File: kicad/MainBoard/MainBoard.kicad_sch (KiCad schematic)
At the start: 97 parts, among them J1 CHAN1, J10 ACC Port, J11 433TX, J12 VDC INPUT, J13 BAT, J14 TRG1, J15 TRG2, J16 FP-BUTTONS, J17 EXPAN2, J18 OUTPUT_BOARD_POWER, J19 FrontPanel, J2 CHAN2, J20 I2C, J21 EXPAN3, J3 OUTPUT_BOARD_IO, J4 OUTPUT_BOARD_FP, J5 CHAN4, J6 LCD, J7 CHAN3, J8 EXPAN1, J9 AudioJack3_SwitchTR, SW1 SW_SPST, U1 AT24C04C-PUM, U2 UT232A, U3 LM2941T, U4 Pico, U5 L78L33ACZTR, U6 LM2576T-5, U7 PCF8574, U8 PCF8574

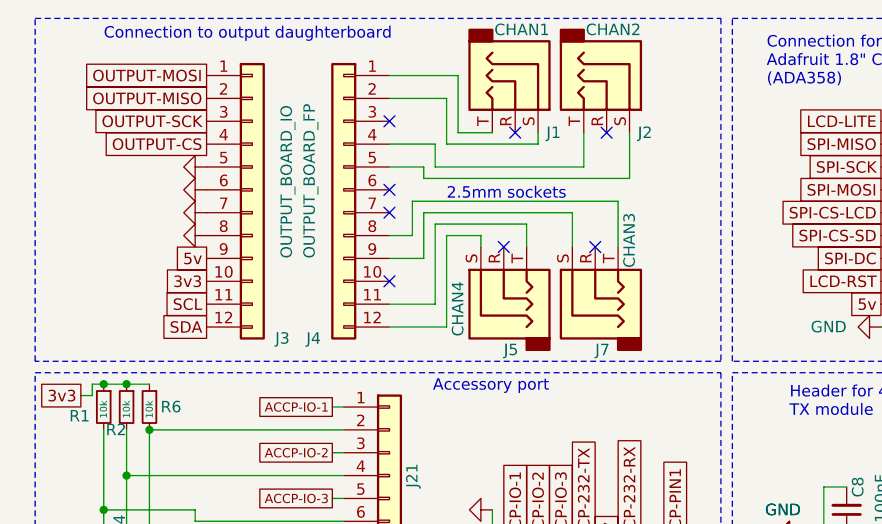
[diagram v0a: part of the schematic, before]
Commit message: Before 3.5mm footprint switch
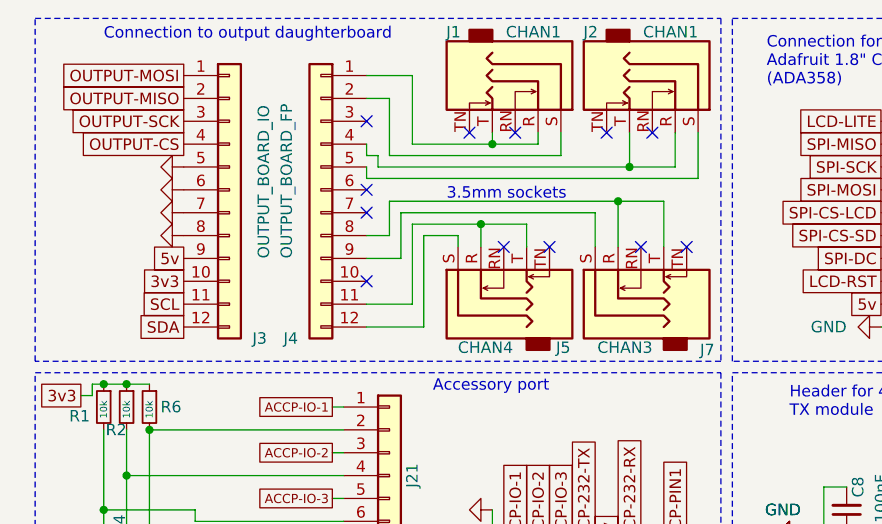
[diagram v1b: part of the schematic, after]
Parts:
- removed J1: CHAN1, ProjLib:PJ-2100B-4A, symbol MainBoard-rescue:AudioJack3-Connector
- removed J2: CHAN2, ProjLib:PJ-2100B-4A, symbol MainBoard-rescue:AudioJack3-Connector
- removed J5: CHAN4, ProjLib:PJ-2100B-4A, symbol MainBoard-rescue:AudioJack3-Connector
- removed J7: CHAN3, ProjLib:PJ-2100B-4A, symbol MainBoard-rescue:AudioJack3-Connector
- added J1, J2: CHAN1, ProjLib:PJ-3062-CO, symbol MainBoard-rescue:AudioJack3_SwitchTR-Connector
- added J5: CHAN4, ProjLib:PJ-3062-CO, symbol MainBoard-rescue:AudioJack3_SwitchTR-Connector
- added J7: CHAN3, ProjLib:PJ-3062-CO, symbol MainBoard-rescue:AudioJack3_SwitchTR-Connector
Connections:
- net at J4.1 (Pin_1): now also J1.R, J1.T
- net at J4.11 (Pin_11): now also J5.R, J5.T
- net at J4.12 (Pin_12): now also J5.S
- net at J4.2 (Pin_2): now also J1.S
- net at J4.4 (Pin_4): now also J2.R, J2.T
- net at J4.5 (Pin_5): now also J2.S
- net at J4.8 (Pin_8): now also J7.R, J7.T
- net at J4.9 (Pin_9): now also J7.S
- no-connect marks 29 -> 33
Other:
- note removed: "2.5mm sockets"
- moved on the sheet: J3, J4
